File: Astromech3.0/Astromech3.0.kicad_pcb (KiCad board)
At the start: 2 copper layers, 32.3 x 50 mm, 48 parts, among them J1 Screw_Terminal_01x02, J2 Conn_01x04, J3 USB_B_Micro, J4 Conn_01x03_Male, J5 Conn_01x05, SW1 SW_Push, SW2 SW_Push, U1 STM32F103C8Tx, U2 MPU-6050, U3 AMS1117, U4 W25Q128JVS, Y1 Crystal

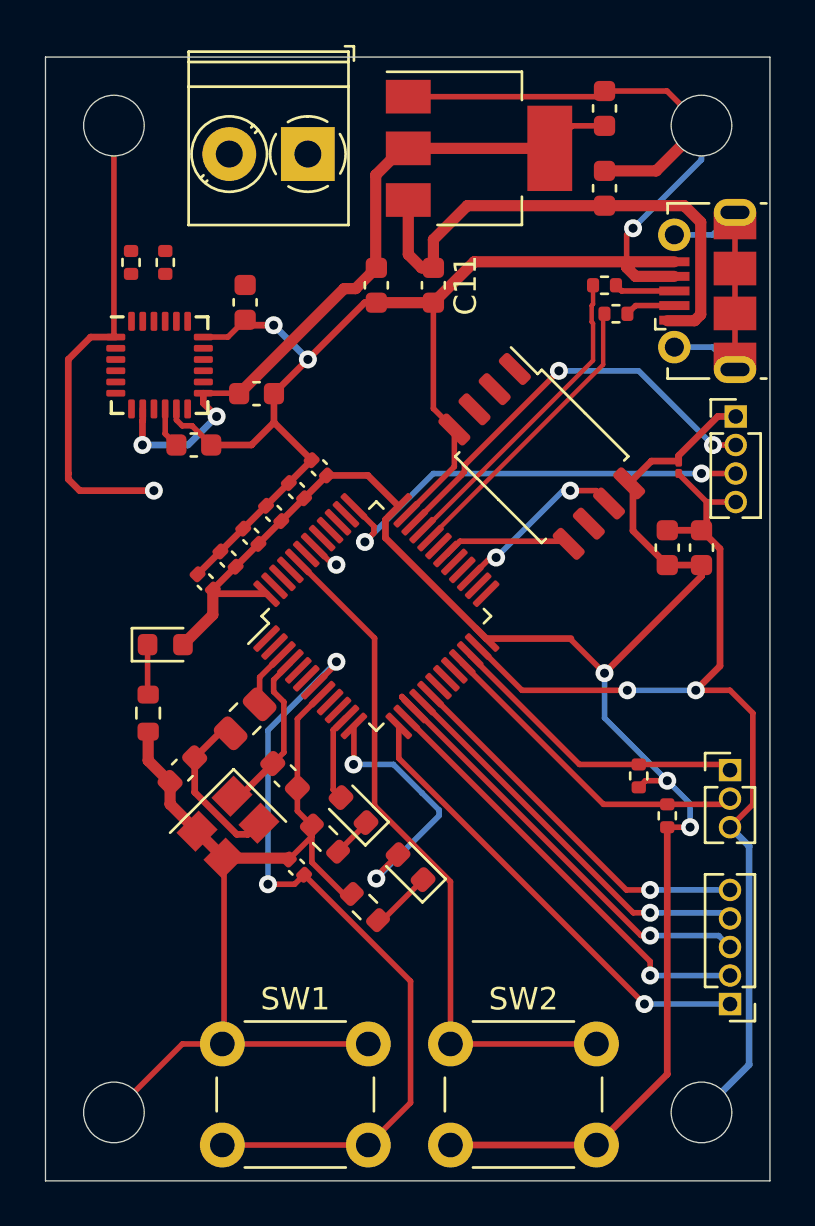
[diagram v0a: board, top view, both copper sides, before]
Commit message: final manufactured board
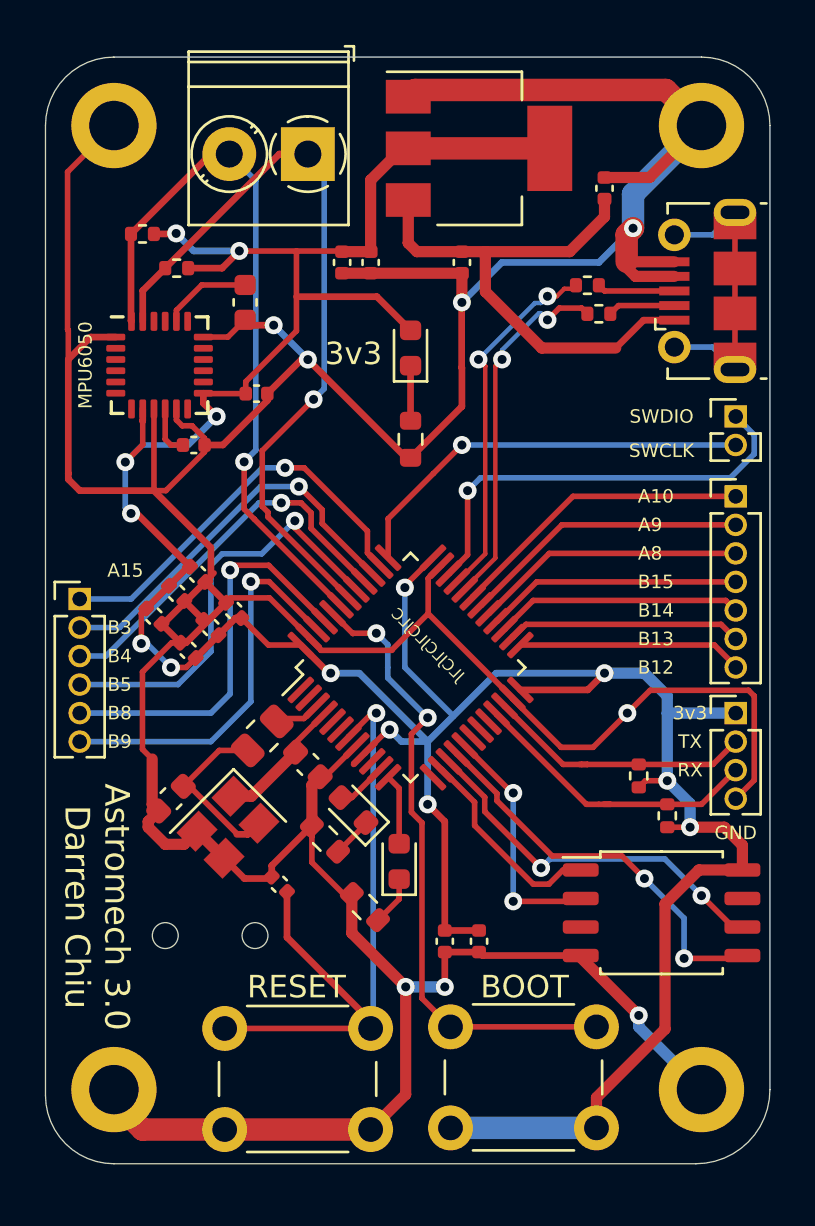
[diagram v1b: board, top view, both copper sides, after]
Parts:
- removed C14: 100uF, Capacitor_SMD:C_0603_1608Metric
- added J6: Conn_01x06, Connector_PinHeader_1.27mm:PinHeader_1x06_P1.27mm_Vertical, F.Cu at (152.1, 78.2)
- C11: value 100uF -> 100nF; footprint Capacitor_SMD:C_0603_1608Metric -> Capacitor_SMD:C_0402_1005Metric
- C12, C13, C15, C18, C19: footprint Capacitor_SMD:C_0603_1608Metric -> Capacitor_SMD:C_0402_1005Metric
- C17: value 100nF -> 10uF; footprint Capacitor_SMD:C_0603_1608Metric -> Capacitor_SMD:C_0402_1005Metric
- C8: value 1uF -> 10uF; footprint Capacitor_SMD:C_01005_0402Metric -> Capacitor_SMD:C_0402_1005Metric
- H1, H2, H3, H4: footprint MountingHole:MountingHole_2.7mm_M2.5 -> MountingHole:MountingHole_2.2mm_M2_DIN965_Pad
- J2: value Conn_01x04 -> Conn_01x02; footprint Connector_PinHeader_1.27mm:PinHeader_1x04_P1.27mm_Vertical -> Connector_PinHeader_1.27mm:PinHeader_1x02_P1.27mm_Vertical
- J4: value Conn_01x03_Male -> Conn_01x04; footprint Connector_PinHeader_1.27mm:PinHeader_1x03_P1.27mm_Vertical -> Connector_PinHeader_1.27mm:PinHeader_1x04_P1.27mm_Vertical
- J5: value Conn_01x05 -> Conn_01x07; footprint Connector_PinHeader_1.27mm:PinHeader_1x05_P1.27mm_Vertical -> Connector_PinHeader_1.27mm:PinHeader_1x07_P1.27mm_Vertical
- moved J5 22.6 mm to (181.4, 73.7), turned to 0 degrees
- moved U4 21.0 mm to (178.1, 92.2), turned to 0 degrees
- moved C18 20.9 mm to (168.4, 93.5), turned to 90 degrees
- moved C19 19.4 mm to (169.9, 93.5), turned to 90 degrees
- moved D1 17.1 mm to (166.9, 67.1), turned to 90 degrees
- moved R6 16.9 mm to (166.9, 71.1)
- moved C8 13.3 mm to (169.2, 63.2)
- moved C17 12.5 mm to (165.1, 63.2), turned to 270 degrees
- moved SW1 7.62 mm to (165.1, 101.9), turned to 180 degrees
- moved C7 7.20 mm to (157.4, 77.1), turned to 315 degrees
- moved C6 6.02 mm to (159.0, 78.7)
- moved C5 5.59 mm to (156.5, 78.0), turned to 315 degrees
- moved C1 5.59 mm to (155.4, 79.0), turned to 315 degrees
- moved C11 4.19 mm to (163.8, 63.2)
- moved C4 3.14 mm to (158.0, 79.5)
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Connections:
- net Net-(U1-Pad18) renamed PB0
- net Net-(U1-Pad19) renamed PB1
- net Net-(U1-Pad20) renamed PB2
- C11 pad 1: +5V -> +3V3
- C8 pad 1: +3V3 -> +5V
- J2 pad 1: +3V3 -> SWDIO
- J2 pad 2: SWDIO -> SWCLK
- J4 pad 1: UART_TX -> +3V3
- J4 pad 2: UART_RX -> UART_TX
- J4 pad 3: GND -> UART_RX
- J5 pad 1: PA3 -> PA10
- J5 pad 2: PA4 -> PA9
- J5 pad 3: PA5 -> PA8
- J5 pad 4: PA6 -> PB15
- J5 pad 5: PA7 -> PB14
- U1 pad 13: PA3 -> Net-(U1-Pad13)
- U1 pad 14: PA4 -> QSPI_CS
- U1 pad 15: PA5 -> QSPI_CLK
- U1 pad 16: PA6 -> SPI_MISO
- U1 pad 17: PA7 -> SPI_MOSI
- U1 pad 25: QSPI_CS -> PB12
- U1 pad 26: QSPI_CLK -> PB13
- U1 pad 27: QSPI_IO3 -> PB14
- U1 pad 28: QSPI_IO2 -> PB15
- U1 pad 29: QSPI_IO1 -> PA8
- U1 pad 30: QSPI_IO0 -> PA9
- U1 pad 31: Net-(U1-Pad31) -> PA10
- U1 pad 38: Net-(U1-Pad38) -> PA15
- U1 pad 39: Net-(U1-Pad39) -> PB3
- U1 pad 40: Net-(U1-Pad40) -> PB4
- U1 pad 41: Net-(U1-Pad41) -> PB5
- U1 pad 45: Net-(U1-Pad45) -> PB8
- U1 pad 46: Net-(U1-Pad46) -> PB9
- U4 pad 2: QSPI_IO1 -> SPI_MOSI
- U4 pad 3: QSPI_IO2 -> Net-(U4-Pad3)
- U4 pad 5: QSPI_IO0 -> SPI_MISO
- U4 pad 7: QSPI_IO3 -> Net-(U4-Pad7)
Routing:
- net +3V3: track 113.7 -> 151.1 mm, vias 5 -> 14
- net GND: track 193.7 -> 229.1 mm, vias 6 -> 8
- net I2C_SDA: track 0.00 -> 33.4 mm, vias 0 -> 1
- net I2C_SCL: track 1.33 -> 34.0 mm
- net PA3: track 20.7 -> 0.00 mm, vias 1 -> 0
- net PA5: track 20.1 -> 0.00 mm, vias 1 -> 0
- net PA4: track 19.5 -> 0.00 mm, vias 1 -> 0
- net PB5: track 0.00 -> 19.0 mm, vias 0 -> 1
- net PA15: track 0.00 -> 18.2 mm, vias 0 -> 1
- net PB8: track 0.00 -> 17.9 mm, vias 0 -> 1
- net SPI_MISO: track 0.00 -> 17.8 mm, vias 0 -> 2
- net PA6: track 17.7 -> 0.00 mm, vias 1 -> 0
- net PB3: track 0.00 -> 17.6 mm, vias 0 -> 1
- net PB9: track 0.00 -> 17.5 mm, vias 0 -> 1
- net PB4: track 0.00 -> 17.3 mm, vias 0 -> 1
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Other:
- board size 32.3 x 50 mm -> 32.3 x 49.3 mm
- board text added: "3v3"
- board text added: "A10"
- board text added: "A15"
- board text added: "A8"
- board text added: "A9"
- board text added: "Astromech 3.0 Darren Chiu"
- board text added: "B12"
- board text added: "B13"
- board text added: "B14"
- board text added: "B15"
- board text added: "B3"
- board text added: "B4"
- board text added: "B5"
- board text added: "B8"
- board text added: "B9"
- board text added: "BOOT"
- board text added: "GND"
- board text added: "JLCJLCJLCJLC"
- board text added: "MPU6050"
- board text added: "RESET"
- board text added: "RX"
- board text added: "SCL"
- board text added: "SDA"
- board text added: "SWCLK"
- board text added: "SWDIO"
- board text added: "TX"
